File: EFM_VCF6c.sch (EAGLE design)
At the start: 69 parts, among them IC1 LM13700N, Q1 2N3904, Q2 2N3904, Q3 2N3904, Q4 2N3904, Q5 2N3906, U1 POWER

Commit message: ready to test cut
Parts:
- R16: device rcl:R-US_0309/12 -> rcl:R-US_0207/7
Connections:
- net +12V renamed N$38
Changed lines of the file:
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@@
 <part name="R17" library="rcl" deviceset="R-US_" device="0207/7" value="1k"/>
 <part name="GND10" library="supply1" deviceset="GND" device=""/>
-<part name="R16" library="rcl" deviceset="R-US_" device="0309/12" value="10k"/>
+<part name="R16" library="rcl" deviceset="R-US_" device="0207/7" value="10k"/>
 <part name="P+7" library="supply1" deviceset="+12V" device=""/>
 <part name="P-5" library="supply1" deviceset="-12V" device=""/>
@@
 </segment>
 </net>
-<net name="+12V" class="0">
+<net name="N$38" class="0">
 <segment>
 <pinref part="U1" gate="G$1" pin="+12V"/>

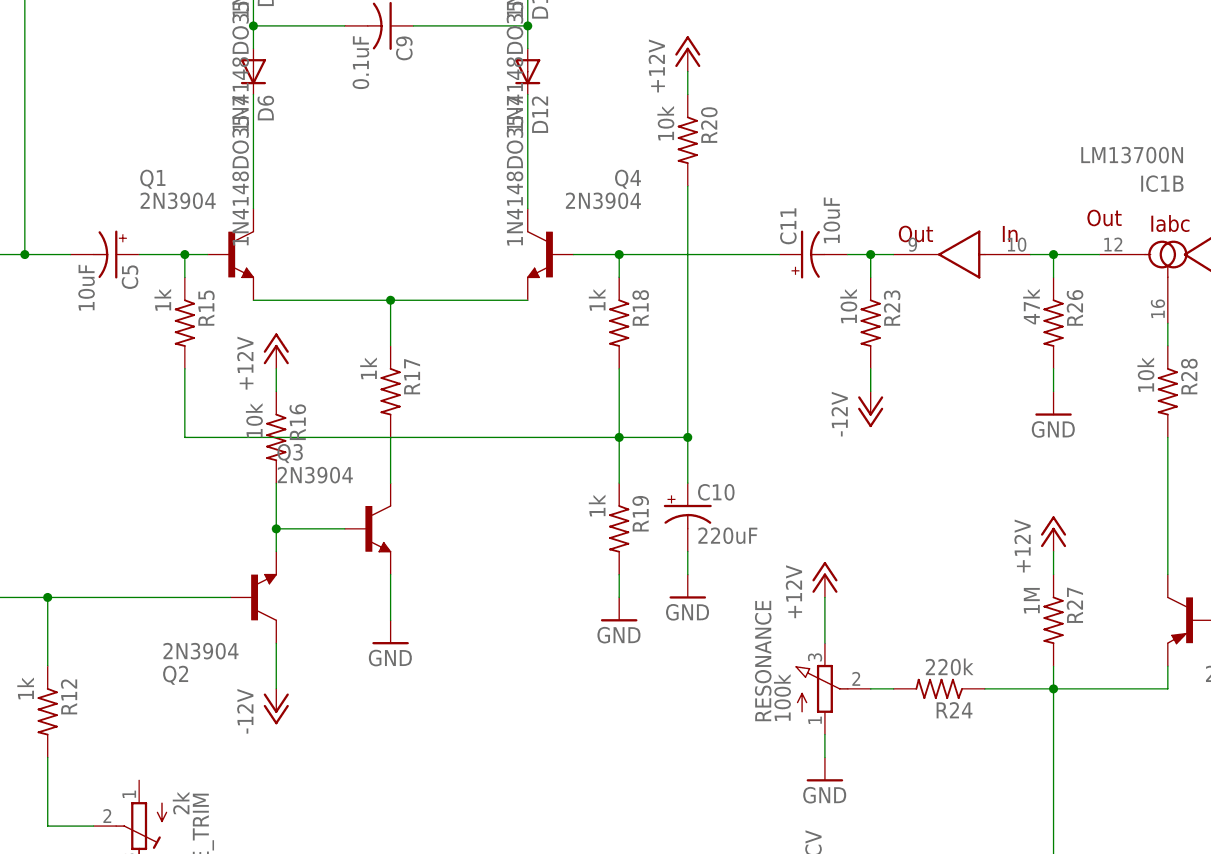
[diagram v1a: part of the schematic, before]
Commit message: fix and mod for self res
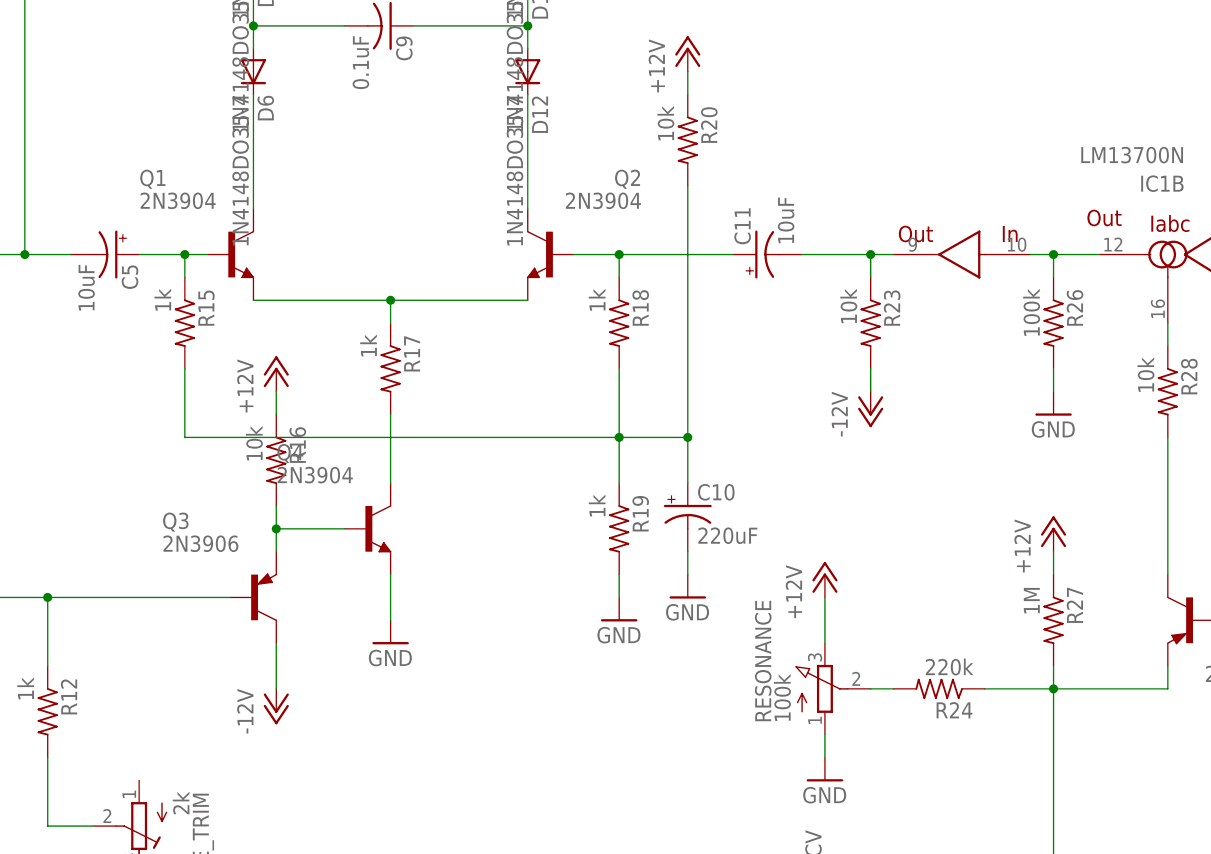
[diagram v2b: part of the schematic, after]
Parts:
- Q3: value 2N3904 -> 2N3906; device transistor-npn:2N3904 -> transistor-pnp:2N3906
- R26: value 47k -> 100k
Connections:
- net -12V: now also Q3.C; no longer Q2.C
- net GND: now also Q4.E; no longer Q3.E
- net N$16: now also Q3.B; no longer Q2.B
- net N$20: now also Q2.C; no longer Q4.C
- net N$26: now also Q2.B; no longer Q4.B
- net N$3: now also Q4.C; no longer Q3.C
- net N$4: now also Q2.E; no longer Q4.E
- net N$8: now also Q3.E, Q4.B; no longer Q2.E, Q3.B
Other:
- moved on the sheet: C11, Q2, Q4, R16, R17
